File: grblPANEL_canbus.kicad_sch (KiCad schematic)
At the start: 14 parts, among them J301 Conn_01x02, U301 SN65HVD230

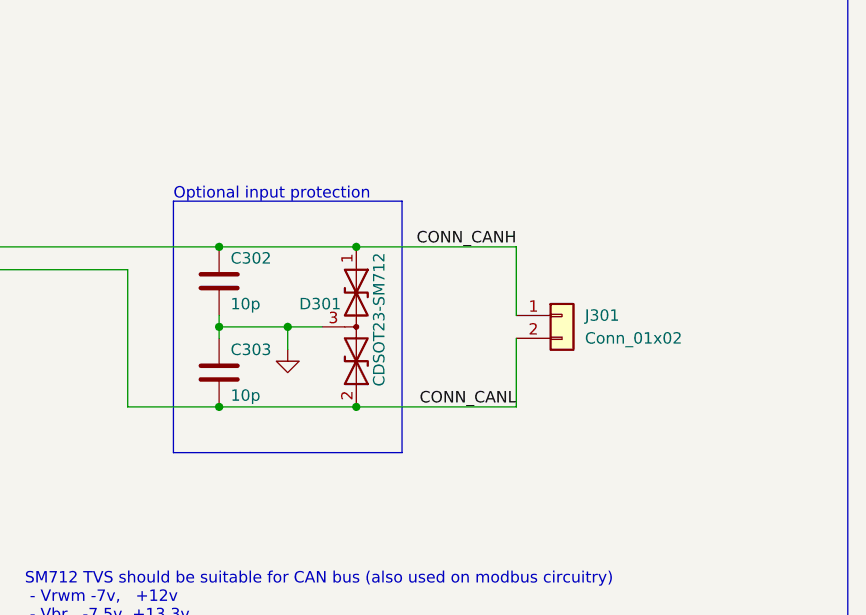
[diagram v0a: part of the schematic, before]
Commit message: small cleanups
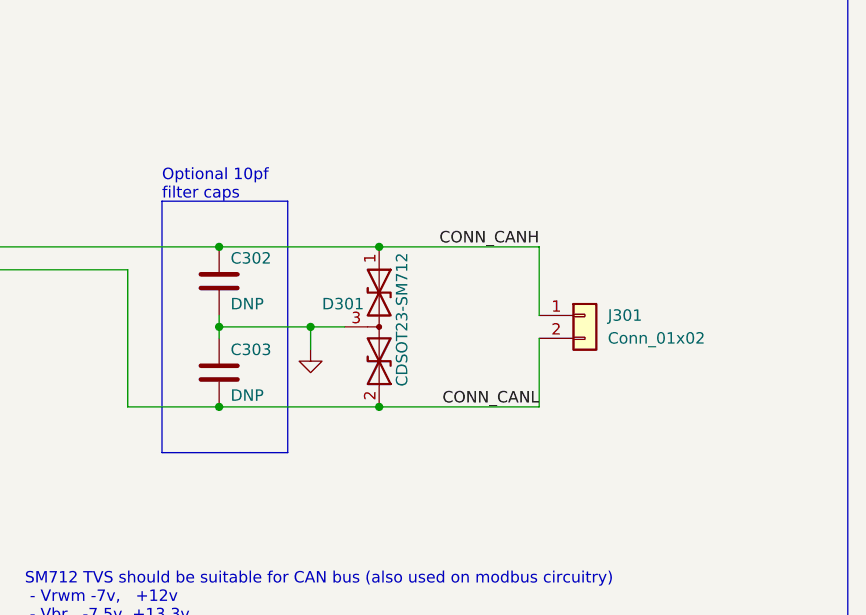
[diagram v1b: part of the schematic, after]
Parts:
- C302, C303: value 10p -> DNP
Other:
- note added: "Optional 10pf filter caps"
- note removed: "Optional input protection"
- moved on the sheet: D301, J301
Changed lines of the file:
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@@
   (junction (at 82.55 86.36) (diameter 0) (color 0 0 0 0)
   )
-  (junction (at 207.01 86.36) (diameter 0) (color 0 0 0 0)
+  (junction (at 209.55 86.36) (diameter 0) (color 0 0 0 0)
   )
   (junction (at 191.77 86.36) (diameter 0) (color 0 0 0 0)
@@
   (junction (at 121.92 71.12) (diameter 0) (color 0 0 0 0)
   )
-  (junction (at 207.01 68.58) (diameter 0) (color 0 0 0 0)
-  )
-  (junction (at 199.39 77.47) (diameter 0) (color 0 0 0 0)
+  (junction (at 209.55 68.58) (diameter 0) (color 0 0 0 0)
+  )
+  (junction (at 201.93 77.47) (diameter 0) (color 0 0 0 0)
   )
   (junction (at 138.43 68.58) (diameter 0) (color 0 0 0 0)
@@
     (stroke (width 0) (type default) (color 0 0 0 0))
   )
-  (polyline (pts (xy 212.09 91.44) (xy 186.69 91.44))
+  (polyline (pts (xy 199.39 91.44) (xy 185.42 91.44))
     (stroke (width 0) (type default) (color 0 0 0 0))
   )
@@
     (stroke (width 0) (type default) (color 0 0 0 0))
   )
-  (polyline (pts (xy 212.09 63.5) (xy 212.09 91.44))
-    (stroke (width 0) (type default) (color 0 0 0 0))
-  )
-  (wire (pts (xy 203.2 77.47) (xy 199.39 77.47))
+  (polyline (pts (xy 199.39 63.5) (xy 199.39 91.44))
+    (stroke (width 0) (type default) (color 0 0 0 0))
+  )
+  (wire (pts (xy 205.74 77.47) (xy 201.93 77.47))
     (stroke (width 0) (type default) (color 0 0 0 0))
   )
@@
     (stroke (width 0) (type default) (color 0 0 0 0))
   )
-  (wire (pts (xy 191.77 68.58) (xy 207.01 68.58))
-    (stroke (width 0) (type default) (color 0 0 0 0))
-  )
-  (polyline (pts (xy 186.69 63.5) (xy 212.09 63.5))
+  (wire (pts (xy 191.77 68.58) (xy 209.55 68.58))
+    (stroke (width 0) (type default) (color 0 0 0 0))
+  )
+  (polyline (pts (xy 185.42 63.5) (xy 199.39 63.5))
     (stroke (width 0) (type default) (color 0 0 0 0))
   )
@@
     (stroke (width 0) (type default) (color 0 0 0 0))
   )
-  (wire (pts (xy 224.79 78.74) (xy 224.79 86.36))
+  (wire (pts (xy 227.33 78.74) (xy 227.33 86.36))
     (stroke (width 0) (type default) (color 0 0 0 0))
   )
@@
     (stroke (width 0) (type default) (color 0 0 0 0))
   )
-  (polyline (pts (xy 186.69 63.5) (xy 186.69 91.44))
+  (polyline (pts (xy 185.42 63.5) (xy 185.42 91.44))
     (stroke (width 0) (type default) (color 0 0 0 0))
   )
@@
     (stroke (width 0) (type default) (color 0 0 0 0))
   )
-  (wire (pts (xy 199.39 77.47) (xy 191.77 77.47))
+  (wire (pts (xy 201.93 77.47) (xy 191.77 77.47))
     (stroke (width 0) (type default) (color 0 0 0 0))
   )
@@
     (stroke (width 0) (type default) (color 0 0 0 0))
   )
-  (wire (pts (xy 207.01 86.36) (xy 191.77 86.36))
+  (wire (pts (xy 209.55 86.36) (xy 191.77 86.36))
     (stroke (width 0) (type default) (color 0 0 0 0))
   )
@@
     (stroke (width 0) (type default) (color 0 0 0 0))
   )
-  (wire (pts (xy 224.79 76.2) (xy 224.79 68.58))
+  (wire (pts (xy 227.33 76.2) (xy 227.33 68.58))
     (stroke (width 0) (type default) (color 0 0 0 0))
   )
@@
     (stroke (width 0) (type default) (color 0 0 0 0))
   )
-  (wire (pts (xy 207.01 68.58) (xy 224.79 68.58))
+  (wire (pts (xy 209.55 68.58) (xy 227.33 68.58))
     (stroke (width 0) (type default) (color 0 0 0 0))
   )
@@
     (stroke (width 0) (type default) (color 0 0 0 0))
   )
-  (wire (pts (xy 199.39 77.47) (xy 199.39 80.01))
+  (wire (pts (xy 201.93 77.47) (xy 201.93 80.01))
     (stroke (width 0) (type default) (color 0 0 0 0))
   )
@@
     (stroke (width 0) (type default) (color 0 0 0 0))
   )
-  (wire (pts (xy 224.79 86.36) (xy 207.01 86.36))
+  (wire (pts (xy 227.33 86.36) (xy 209.55 86.36))
     (stroke (width 0) (type default) (color 0 0 0 0))
   )
@@
     (effects (font (size 1.27 1.27)) (justify left bottom))
   )
-  (text "Optional input protection" (at 186.69 63.5 0)
+  (text "Optional 10pf\nfilter caps" (at 185.42 63.5 0)
     (effects (font (size 1.27 1.27)) (justify left bottom))
   )
@@
     (effects (font (size 1.27 1.27)) (justify right bottom))
   )
-  (label "CONN_CANH" (at 224.79 68.58 180)
+  (label "CONN_CANH" (at 227.33 68.58 180)
     (effects (font (size 1.27 1.27)) (justify right bottom))
   )
@@
     (effects (font (size 1.27 1.27)) (justify right bottom))
   )
-  (label "CONN_CANL" (at 224.79 86.36 180)
+  (label "CONN_CANL" (at 227.33 86.36 180)
     (effects (font (size 1.27 1.27)) (justify right bottom))
   )
@@
     (pin "1")
   )
-  (symbol (lib_id "Device:D_TVS_Dual_AAC") (at 207.01 77.47 270) (unit 1)
-    (in_bom yes) (on_board yes)
-    (property "Reference" "D301" (id 0) (at 200.66 74.93 90)
-      (effects (font (size 1.27 1.27)) (justify left))
-    )
-    (property "Value" "CDSOT23-SM712" (id 1) (at 209.55 69.215 0)
-      (effects (font (size 1.27 1.27)) (justify left))
-    )
-    (property "Footprint" "Package_TO_SOT_SMD:SOT-23" (id 2) (at 207.01 73.66 0)
-      (effects (font (size 1.27 1.27)) hide)
-    )
-    (property "Datasheet" "~" (id 3) (at 207.01 73.66 0)
+  (symbol (lib_id "Device:D_TVS_Dual_AAC") (at 209.55 77.47 270) (unit 1)
+    (in_bom yes) (on_board yes)
+    (property "Reference" "D301" (id 0) (at 203.2 74.93 90)
+      (effects (font (size 1.27 1.27)) (justify left))
+    )
+    (property "Value" "CDSOT23-SM712" (id 1) (at 212.09 69.215 0)
+      (effects (font (size 1.27 1.27)) (justify left))
+    )
+    (property "Footprint" "Package_TO_SOT_SMD:SOT-23" (id 2) (at 209.55 73.66 0)
+      (effects (font (size 1.27 1.27)) hide)
+    )
+    (property "Datasheet" "~" (id 3) (at 209.55 73.66 0)
       (effects (font (size 1.27 1.27)) hide)
     )
@@
     (pin "2")
   )
-  (symbol (lib_id "Connector_Generic:Conn_01x02") (at 229.87 76.2 0) (unit 1)
+  (symbol (lib_id "Connector_Generic:Conn_01x02") (at 232.41 76.2 0) (unit 1)
     (in_bom yes) (on_board yes) (fields_autoplaced)
-    (property "Reference" "J301" (id 0) (at 232.41 76.1999 0)
-      (effects (font (size 1.27 1.27)) (justify left))
-    )
-    (property "Value" "Conn_01x02" (id 1) (at 232.41 78.7399 0)
-      (effects (font (size 1.27 1.27)) (justify left))
-    )
-    (property "Footprint" "TerminalBlock_Phoenix:TerminalBlock_Phoenix_PT-1,5-2-3.5-H_1x02_P3.50mm_Horizontal" (id 2) (at 229.87 76.2 0)
-      (effects (font (size 1.27 1.27)) hide)
-    )
-    (property "Datasheet" "~" (id 3) (at 229.87 76.2 0)
-      (effects (font (size 1.27 1.27)) hide)
-    )
-    (pin "1")
-    (pin "2")
-  )
-  (symbol (lib_id "power:GND") (at 199.39 80.01 0) (unit 1)
-    (in_bom yes) (on_board yes)
-    (property "Reference" "#PWR0304" (id 0) (at 199.39 86.36 0)
-      (effects (font (size 1.27 1.27)) hide)
-    )
-    (property "Value" "GND" (id 1) (at 200.66 83.82 0)
-      (effects (font (size 1.27 1.27)) hide)
-    )
-    (property "Footprint" "" (id 2) (at 199.39 80.01 0)
-      (effects (font (size 1.27 1.27)) hide)
-    )
-    (property "Datasheet" "" (id 3) (at 199.39 80.01 0)
+    (property "Reference" "J301" (id 0) (at 234.95 76.1999 0)
+      (effects (font (size 1.27 1.27)) (justify left))
+    )
+    (property "Value" "Conn_01x02" (id 1) (at 234.95 78.7399 0)
+      (effects (font (size 1.27 1.27)) (justify left))
+    )
+    (property "Footprint" "TerminalBlock_Phoenix:TerminalBlock_Phoenix_PT-1,5-2-3.5-H_1x02_P3.50mm_Horizontal" (id 2) (at 232.41 76.2 0)
+      (effects (font (size 1.27 1.27)) hide)
+    )
+    (property "Datasheet" "~" (id 3) (at 232.41 76.2 0)
+      (effects (font (size 1.27 1.27)) hide)
+    )
+    (pin "1")
+    (pin "2")
+  )
+  (symbol (lib_id "power:GND") (at 201.93 80.01 0) (unit 1)
+    (in_bom yes) (on_board yes)
+    (property "Reference" "#PWR0304" (id 0) (at 201.93 86.36 0)
+      (effects (font (size 1.27 1.27)) hide)
+    )
+    (property "Value" "GND" (id 1) (at 203.2 83.82 0)
+      (effects (font (size 1.27 1.27)) hide)
+    )
+    (property "Footprint" "" (id 2) (at 201.93 80.01 0)
+      (effects (font (size 1.27 1.27)) hide)
+    )
+    (property "Datasheet" "" (id 3) (at 201.93 80.01 0)
       (effects (font (size 1.27 1.27)) hide)
     )
@@
       (effects (font (size 1.27 1.27)) (justify left))
     )
-    (property "Value" "10p" (id 1) (at 193.04 85.09 0)
+    (property "Value" "DNP" (id 1) (at 193.04 85.09 0)
       (effects (font (size 1.27 1.27)) (justify left))
     )
@@
       (effects (font (size 1.27 1.27)) (justify left))
     )
-    (property "Value" "10p" (id 1) (at 193.04 74.93 0)
-      (effects (font (size 1.27 1.27)) (justify left))
-    )
+    (property "Value" "DNP" (id 1) (at 193.04 74.93 0)
+      (effects (font (size 1.27 1.27)) (justify left))
+    )
